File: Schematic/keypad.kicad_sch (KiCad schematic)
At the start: 9 parts, among them J2 Conn_01x08

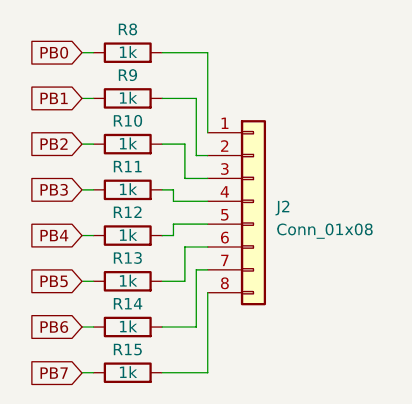
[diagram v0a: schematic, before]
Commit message: initial CB design
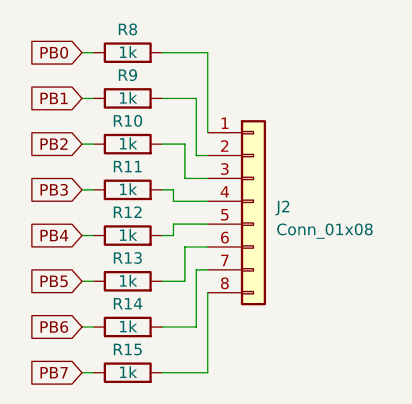
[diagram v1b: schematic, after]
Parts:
- R10, R11, R12, R13, R14, R15, R8, R9: footprint Resistor_SMD:R_0805_2012Metric_Pad1.20x1.40mm_HandSolder -> Resistor_SMD:R_1206_3216Metric_Pad1.30x1.75mm_HandSolder
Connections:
- net PB7: now also R15.1
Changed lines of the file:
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@@
+    (stroke (width 0) (type default))
+  )
+  (wire (pts (xy 40.64 43.18) (xy 41.91 43.18))
+    (stroke (width 0) (type default))
+  )
+  (wire (pts (xy 40.64 49.53) (xy 40.64 43.18))
+    (stroke (width 0) (type default))
+  )
+  (wire (pts (xy 27.94 44.45) (xy 29.21 44.45))
+    (stroke (width 0) (type default))
+  )
+  (wire (pts (xy 27.94 34.29) (xy 29.21 34.29))
+    (stroke (width 0) (type default))
+  )
+  (wire (pts (xy 40.64 30.48) (xy 41.91 30.48))
+    (stroke (width 0) (type default))
+  )
+  (wire (pts (xy 36.83 19.05) (xy 41.91 19.05))
+    (stroke (width 0) (type default))
+  )
+  (wire (pts (xy 38.1 35.56) (xy 38.1 34.29))
+    (stroke (width 0) (type default))
+  )
+  (wire (pts (xy 39.37 29.21) (xy 39.37 33.02))
+    (stroke (width 0) (type default))
+  )
+  (wire (pts (xy 27.94 29.21) (xy 29.21 29.21))
+    (stroke (width 0) (type default))
+  )
+  (wire (pts (xy 27.94 39.37) (xy 29.21 39.37))
+    (stroke (width 0) (type default))
+  )
+  (wire (pts (xy 40.64 24.13) (xy 40.64 30.48))
+    (stroke (width 0) (type default))
+  )
+  (wire (pts (xy 38.1 35.56) (xy 41.91 35.56))
+    (stroke (width 0) (type default))
+  )
+  (wire (pts (xy 38.1 39.37) (xy 38.1 38.1))
+    (stroke (width 0) (type default))
+  )
+  (wire (pts (xy 36.83 54.61) (xy 41.91 54.61))
+    (stroke (width 0) (type default))
+  )
+  (wire (pts (xy 38.1 34.29) (xy 36.83 34.29))
+    (stroke (width 0) (type default))
+  )
+  (wire (pts (xy 27.94 24.13) (xy 29.21 24.13))
+    (stroke (width 0) (type default))
+  )
+  (wire (pts (xy 27.94 19.05) (xy 29.21 19.05))
+    (stroke (width 0) (type default))
+  )
+  (wire (pts (xy 36.83 44.45) (xy 39.37 44.45))
+    (stroke (width 0) (type default))
+  )
+  (wire (pts (xy 41.91 54.61) (xy 41.91 45.72))
+    (stroke (width 0) (type default))
+  )
+  (wire (pts (xy 27.94 49.53) (xy 29.21 49.53))
+    (stroke (width 0) (type default))
+  )
+  (wire (pts (xy 41.91 27.94) (xy 41.91 19.05))
+    (stroke (width 0) (type default))
+  )
+  (wire (pts (xy 36.83 24.13) (xy 40.64 24.13))
+    (stroke (width 0) (type default))
+  )
+  (wire (pts (xy 38.1 38.1) (xy 41.91 38.1))
+    (stroke (width 0) (type default))
+  )
+  (wire (pts (xy 36.83 39.37) (xy 38.1 39.37))
+    (stroke (width 0) (type default))
+  )
+  (wire (pts (xy 36.83 49.53) (xy 40.64 49.53))
+    (stroke (width 0) (type default))
+  )
+  (wire (pts (xy 36.83 29.21) (xy 39.37 29.21))
     (stroke (width 0) (type default))
   )
@@
     (stroke (width 0) (type default))
   )
-  (wire (pts (xy 40.64 43.18) (xy 41.91 43.18))
-    (stroke (width 0) (type default))
-  )
-  (wire (pts (xy 40.64 49.53) (xy 40.64 43.18))
-    (stroke (width 0) (type default))
-  )
-  (wire (pts (xy 27.94 44.45) (xy 29.21 44.45))
-    (stroke (width 0) (type default))
-  )
-  (wire (pts (xy 27.94 34.29) (xy 29.21 34.29))
-    (stroke (width 0) (type default))
-  )
-  (wire (pts (xy 40.64 30.48) (xy 41.91 30.48))
-    (stroke (width 0) (type default))
-  )
-  (wire (pts (xy 36.83 19.05) (xy 41.91 19.05))
-    (stroke (width 0) (type default))
-  )
-  (wire (pts (xy 38.1 35.56) (xy 38.1 34.29))
-    (stroke (width 0) (type default))
-  )
-  (wire (pts (xy 39.37 29.21) (xy 39.37 33.02))
-    (stroke (width 0) (type default))
-  )
-  (wire (pts (xy 27.94 29.21) (xy 29.21 29.21))
-    (stroke (width 0) (type default))
-  )
-  (wire (pts (xy 27.94 39.37) (xy 29.21 39.37))
-    (stroke (width 0) (type default))
-  )
-  (wire (pts (xy 40.64 24.13) (xy 40.64 30.48))
-    (stroke (width 0) (type default))
-  )
-  (wire (pts (xy 38.1 35.56) (xy 41.91 35.56))
-    (stroke (width 0) (type default))
-  )
-  (wire (pts (xy 38.1 39.37) (xy 38.1 38.1))
-    (stroke (width 0) (type default))
-  )
-  (wire (pts (xy 36.83 54.61) (xy 41.91 54.61))
-    (stroke (width 0) (type default))
-  )
-  (wire (pts (xy 38.1 34.29) (xy 36.83 34.29))
-    (stroke (width 0) (type default))
-  )
-  (wire (pts (xy 27.94 24.13) (xy 29.21 24.13))
-    (stroke (width 0) (type default))
-  )
-  (wire (pts (xy 27.94 19.05) (xy 29.21 19.05))
-    (stroke (width 0) (type default))
-  )
-  (wire (pts (xy 36.83 44.45) (xy 39.37 44.45))
-    (stroke (width 0) (type default))
-  )
-  (wire (pts (xy 41.91 54.61) (xy 41.91 45.72))
-    (stroke (width 0) (type default))
-  )
-  (wire (pts (xy 27.94 49.53) (xy 29.21 49.53))
-    (stroke (width 0) (type default))
-  )
-  (wire (pts (xy 41.91 27.94) (xy 41.91 19.05))
-    (stroke (width 0) (type default))
-  )
-  (wire (pts (xy 36.83 24.13) (xy 40.64 24.13))
-    (stroke (width 0) (type default))
-  )
-  (wire (pts (xy 38.1 38.1) (xy 41.91 38.1))
-    (stroke (width 0) (type default))
-  )
-  (wire (pts (xy 36.83 39.37) (xy 38.1 39.37))
-    (stroke (width 0) (type default))
-  )
-  (wire (pts (xy 36.83 49.53) (xy 40.64 49.53))
-    (stroke (width 0) (type default))
-  )
-  (wire (pts (xy 36.83 29.21) (xy 39.37 29.21))
-    (stroke (width 0) (type default))
-  )
   (wire (pts (xy 39.37 33.02) (xy 41.91 33.02))
     (stroke (width 0) (type default))
@@
     (stroke (width 0) (type default))
   )
-  (global_label "PB7" (shape input) (at 27.94 54.6504 180) (fields_autoplaced)
-    (effects (font (size 1.27 1.27)) (justify right))
-    (property "Intersheetrefs" "${INTERSHEET_REFS}" (at 21.2847 54.6504 0)
+  (global_label "PB7" (shape input) (at 27.94 54.61 180) (fields_autoplaced)
+    (effects (font (size 1.27 1.27)) (justify right))
+    (property "Intersheetrefs" "${INTERSHEET_REFS}" (at 21.2847 54.61 0)
       (effects (font (size 1.27 1.27)) (justify right) hide)
     )
@@
       (effects (font (size 1.27 1.27)))
     )
-    (property "Footprint" "Resistor_SMD:R_0805_2012Metric_Pad1.20x1.40mm_HandSolder" (at 33.02 41.148 90)
+    (property "Footprint" "Resistor_SMD:R_1206_3216Metric_Pad1.30x1.75mm_HandSolder" (at 33.02 41.148 90)
       (effects (font (size 1.27 1.27)) hide)
     )
@@
       (effects (font (size 1.27 1.27)))
     )
-    (property "Footprint" "Resistor_SMD:R_0805_2012Metric_Pad1.20x1.40mm_HandSolder" (at 33.02 51.308 90)
+    (property "Footprint" "Resistor_SMD:R_1206_3216Metric_Pad1.30x1.75mm_HandSolder" (at 33.02 51.308 90)
       (effects (font (size 1.27 1.27)) hide)
     )
@@
       (effects (font (size 1.27 1.27)))
     )
-    (property "Footprint" "Resistor_SMD:R_0805_2012Metric_Pad1.20x1.40mm_HandSolder" (at 33.02 25.908 90)
+    (property "Footprint" "Resistor_SMD:R_1206_3216Metric_Pad1.30x1.75mm_HandSolder" (at 33.02 25.908 90)
       (effects (font (size 1.27 1.27)) hide)
     )
@@
       (effects (font (size 1.27 1.27)))
     )
-    (property "Footprint" "Resistor_SMD:R_0805_2012Metric_Pad1.20x1.40mm_HandSolder" (at 33.02 20.828 90)
+    (property "Footprint" "Resistor_SMD:R_1206_3216Metric_Pad1.30x1.75mm_HandSolder" (at 33.02 20.828 90)
       (effects (font (size 1.27 1.27)) hide)
     )
@@
       (effects (font (size 1.27 1.27)))
     )
-    (property "Footprint" "Resistor_SMD:R_0805_2012Metric_Pad1.20x1.40mm_HandSolder" (at 33.02 36.068 90)
+    (property "Footprint" "Resistor_SMD:R_1206_3216Metric_Pad1.30x1.75mm_HandSolder" (at 33.02 36.068 90)
       (effects (font (size 1.27 1.27)) hide)
     )
@@
       (effects (font (size 1.27 1.27)))
     )
-    (property "Footprint" "Resistor_SMD:R_0805_2012Metric_Pad1.20x1.40mm_HandSolder" (at 33.02 30.988 90)
+    (property "Footprint" "Resistor_SMD:R_1206_3216Metric_Pad1.30x1.75mm_HandSolder" (at 33.02 30.988 90)
       (effects (font (size 1.27 1.27)) hide)
     )
@@
       (effects (font (size 1.27 1.27)))
     )
-    (property "Footprint" "Resistor_SMD:R_0805_2012Metric_Pad1.20x1.40mm_HandSolder" (at 33.02 46.228 90)
+    (property "Footprint" "Resistor_SMD:R_1206_3216Metric_Pad1.30x1.75mm_HandSolder" (at 33.02 46.228 90)
       (effects (font (size 1.27 1.27)) hide)
     )
@@
       (effects (font (size 1.27 1.27)))
     )
-    (property "Footprint" "Resistor_SMD:R_0805_2012Metric_Pad1.20x1.40mm_HandSolder" (at 33.02 56.388 90)
-      (effects (font (size 1.27 1.27)) hide)
-    )
+    (property "Footprint" "Resistor_SMD:R_1206_3216Metric_Pad1.30x1.75mm_HandSolder" (at 33.02 56.388 90)
+      (effects (font (size 1.27 1.27)) hide)
+    )
